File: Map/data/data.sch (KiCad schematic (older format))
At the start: 0 parts

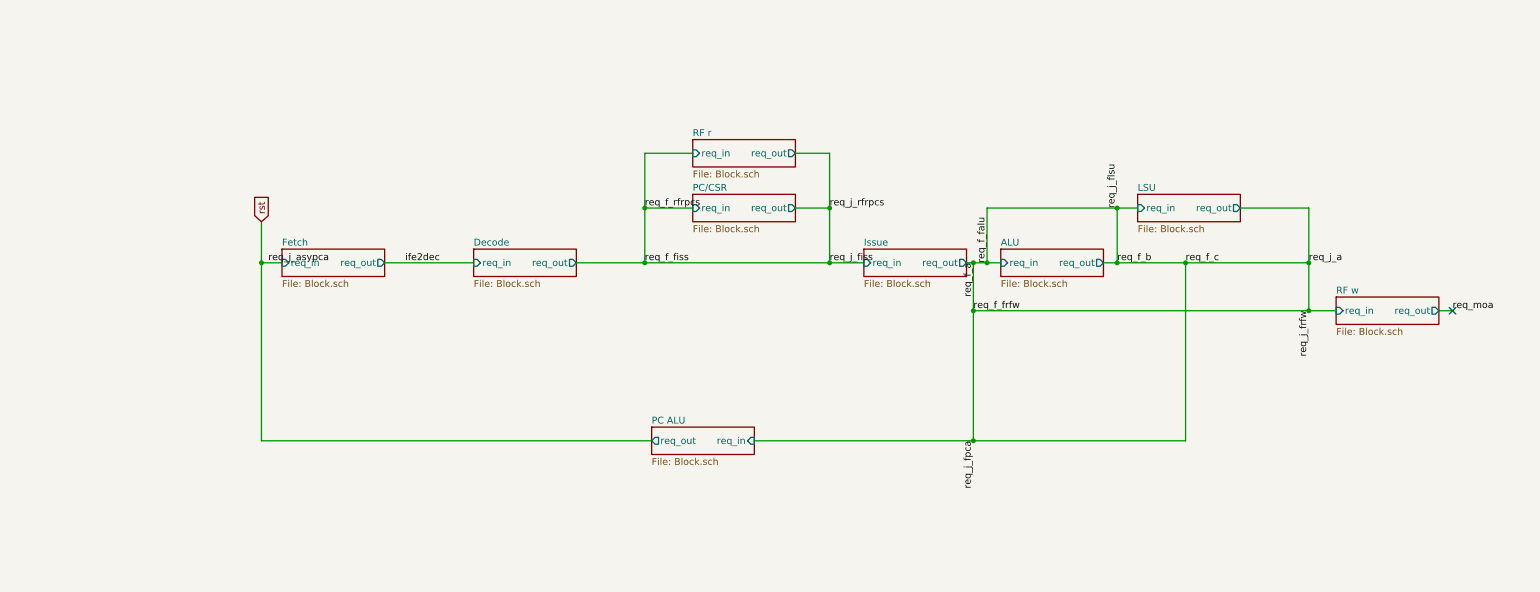
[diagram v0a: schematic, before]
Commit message: travail sur muller
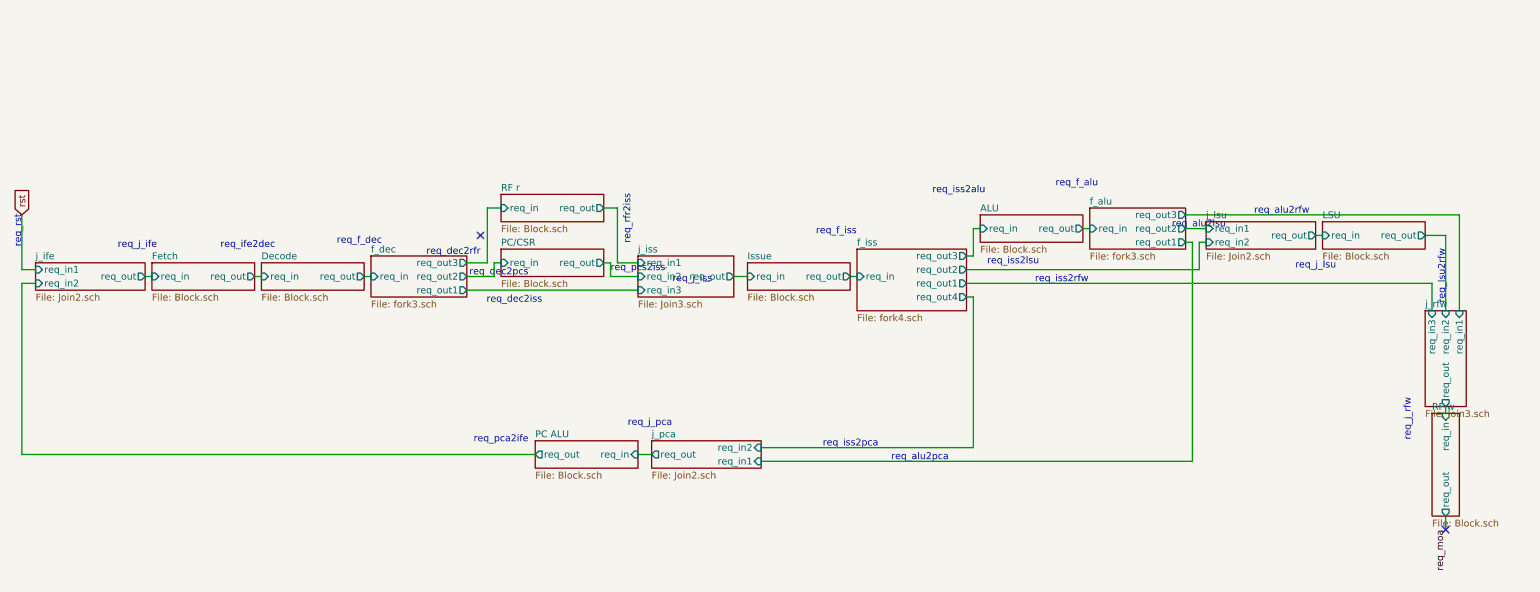
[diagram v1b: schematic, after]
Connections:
- no-connect marks 1 -> 2
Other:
- note added: "req_alu2lsu\n"
- note added: "req_alu2pca"
- note added: "req_alu2rfw\n"
- note added: "req_dec2iss\n"
- note added: "req_dec2pcs\n"
- note added: "req_dec2rfr\n"
- note added: "req_f_alu\n"
- note added: "req_f_dec\n\n"
- note added: "req_f_iss\n"
- note added: "req_ife2dec\n"
- note added: "req_iss2alu\n"
- note added: "req_iss2lsu\n\n"
- note added: "req_iss2pca\n"
- note added: "req_iss2rfw\n"
- note added: "req_j_ife\n"
- note added: "req_j_iss"
- note added: "req_j_lsu\n"
- note added: "req_j_pca\n"
- note added: "req_j_rfw\n"
- note added: "req_lsu2rfw\n"
- note added: "req_pca2ife\n\n"
- note added: "req_pcs2iss\n\n"
- note added: "req_rfr2iss"
- note added: "req_rst\n"

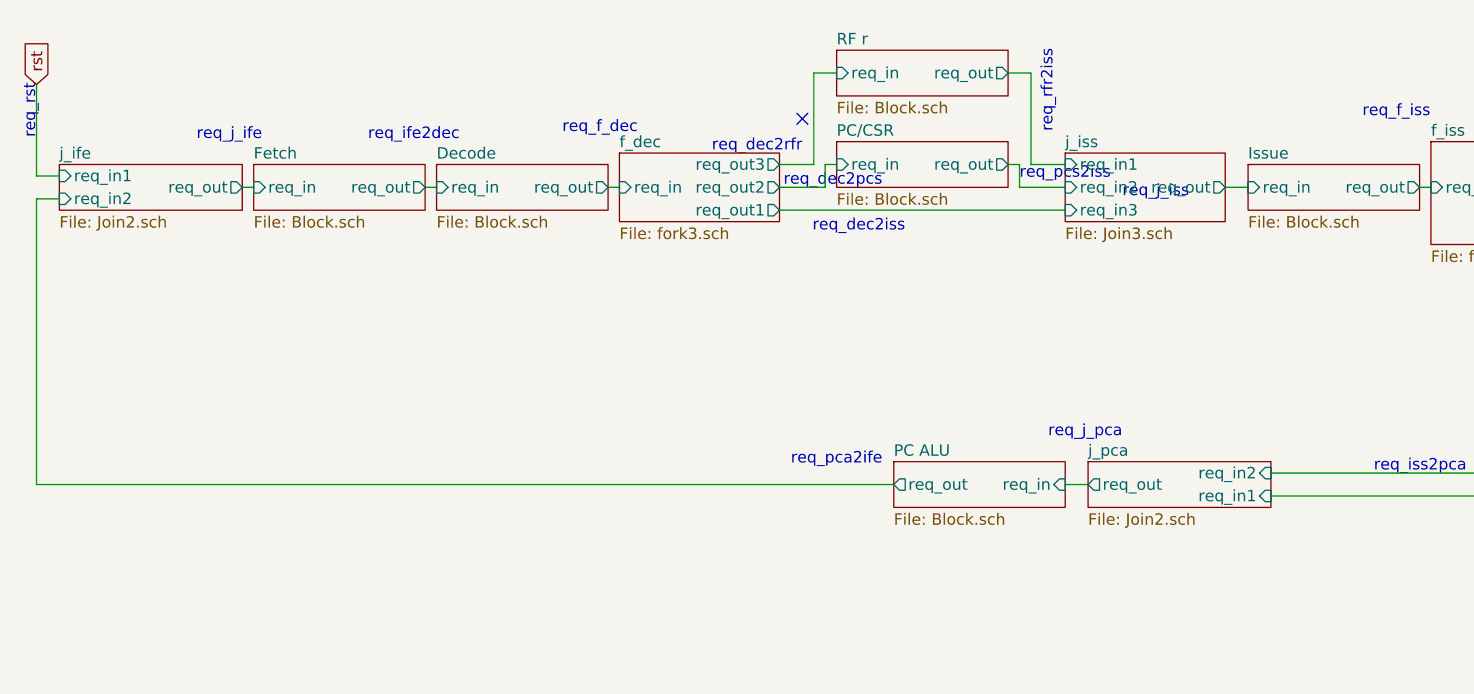
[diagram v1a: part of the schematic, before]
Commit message: Release v1
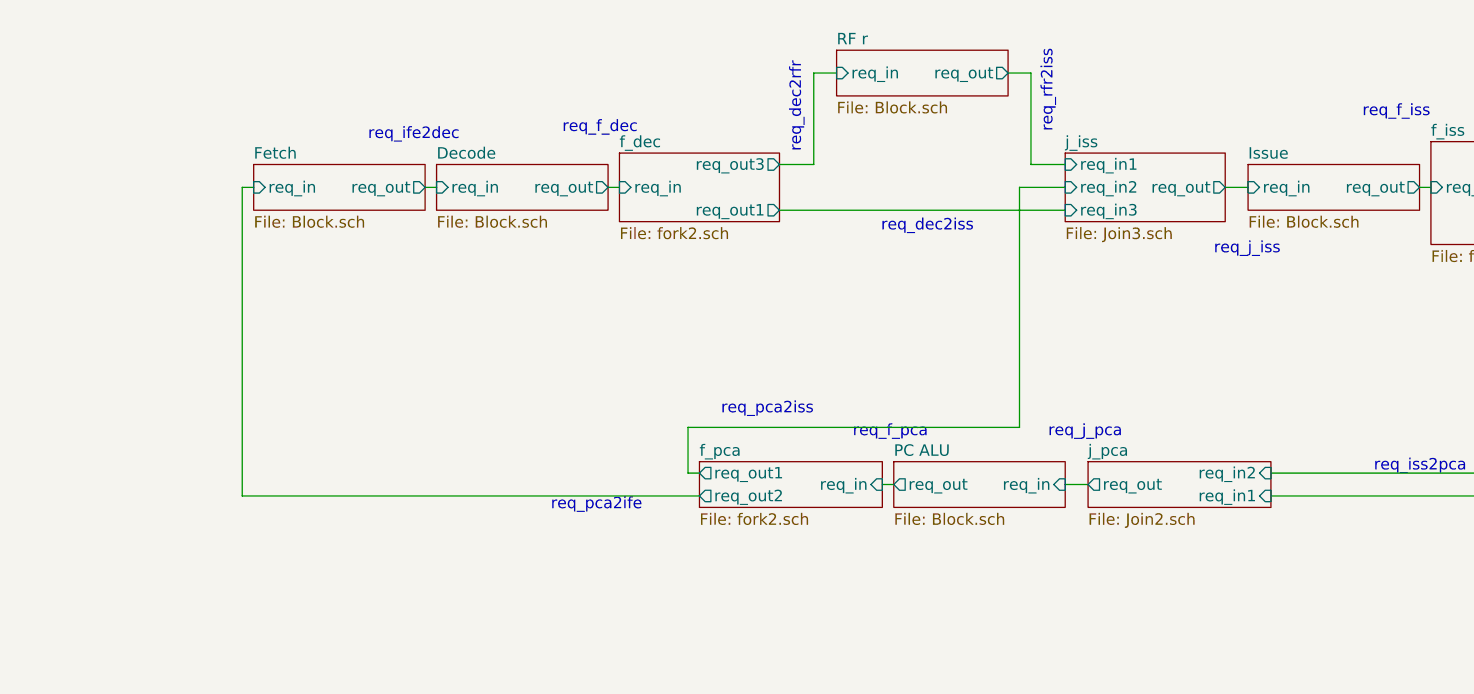
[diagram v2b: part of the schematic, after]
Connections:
- no-connect marks 2 -> 1
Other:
- note added: "req_f_pca"
- note added: "req_pca2iss\n"
- note removed: "req_dec2pcs\n"
- note removed: "req_j_ife\n"
- note removed: "req_pcs2iss\n\n"
- note removed: "req_rst\n"
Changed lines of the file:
@@
 $Descr A4 11693 8268
 encoding utf-8
-Sheet 1 18
+Sheet 1 17
 Title ""
 Date ""
@@
 $EndSheet
 $Sheet
-S 4050 2600 750  200
-U 5EAC82B1
-F0 "PC/CSR" 50
-F1 "Block.sch" 50
-F2 "req_in" I L 4050 2700 50
-F3 "req_out" O R 4800 2700 50
-$EndSheet
-$Sheet
 S 5850 2700 750  200
 U 5EAC8327
@@
 Wire Wire Line
 	1450 2800 1500 2800
-Text GLabel 550  2350 1    50   Input ~ 0
-rst
 Text Label 10950 4650 3    50   ~ 0
 req_moa
-$Sheet
-S 650  2700 800  200
-U 5EAD46D6
-F0 "j_ife" 50
-F1 "Join2.sch" 50
-F2 "req_out" O R 1450 2800 50
-F3 "req_in1" I L 650 2750 50
-F4 "req_in2" I L 650 2850 50
-$EndSheet
-Wire Wire Line
-	650  2750 550  2750
-Wire Wire Line
-	550  2350 550  2750
-Wire Wire Line
-	550  4100 550  2850
-Wire Wire Line
-	550  2850 650  2850
-Wire Wire Line
-	550  4100 4300 4100
 $Sheet
 S 5050 2650 700  300
@@
 F4 "req_in2" I L 5050 2800 50
 F5 "req_in3" I L 5050 2900 50
-$EndSheet
-$Sheet
-S 3100 2650 700  300
-U 5EAD914F
-F0 "f_dec" 50
-F1 "fork3.sch" 50
-F2 "req_in" I L 3100 2800 50
-F3 "req_out1" O R 3800 2900 50
-F4 "req_out2" O R 3800 2800 50
-F5 "req_out3" O R 3800 2700 50
 $EndSheet
 $Sheet
@@
 	5050 2900 3800 2900
 Wire Wire Line
-	3800 2800 4000 2800
-Wire Wire Line
-	4000 2800 4000 2700
-Wire Wire Line
-	4000 2700 4050 2700
-Wire Wire Line
-	4800 2700 4850 2700
-Wire Wire Line
-	4850 2700 4850 2800
-Wire Wire Line
 	4850 2800 5050 2800
 Wire Wire Line
@@
 Text Notes 2000 2600 0    50   ~ 0
 req_ife2dec\n
-Text Notes 1250 2600 0    50   ~ 0
-req_j_ife\n
 Text Notes 2850 2650 0    50   ~ 0
 req_f_dec\n\n
-Text Notes 3900 2650 2    50   ~ 0
-req_dec2rfr\n
-Text Notes 4250 2800 2    50   ~ 0
-req_dec2pcs\n
-Text Notes 4350 3000 2    50   ~ 0
+Text Notes 4650 3000 2    50   ~ 0
 req_dec2iss\n
 Text Notes 5000 2200 3    50   ~ 0
 req_rfr2iss
-Text Notes 4850 2850 0    50   ~ 0
-req_pcs2iss\n\n
 Wire Wire Line
 	4900 2700 5050 2700
-Text Notes 5300 2850 0    50   ~ 0
+Text Notes 5700 3100 0    50   ~ 0
 req_j_iss
 Text Notes 6350 2500 0    50   ~ 0
@@
 Text Notes 5300 3900 2    50   ~ 0
 req_j_pca\n
-Text Notes 4250 4100 2    50   ~ 0
+Text Notes 3200 4300 2    50   ~ 0
 req_pca2ife\n\n
-Text Notes 550  2350 3    50   ~ 0
-req_rst\n
 Text Notes 9850 2750 0    50   ~ 0
 req_j_lsu\n
-NoConn ~ 3900 2500
+$Sheet
+S 3450 4000 800  200
+U 5EB0D305
+F0 "f_pca" 50
+F1 "fork2.sch" 50
+F2 "req_in" I R 4250 4100 50
+F3 "req_out1" O L 3450 4050 50
+F4 "req_out2" O L 3450 4150 50
+$EndSheet
+Wire Wire Line
+	4300 4100 4250 4100
+Text Notes 4450 3900 2    50   ~ 0
+req_f_pca
+Wire Wire Line
+	3450 4150 1450 4150
+Wire Wire Line
+	1450 4150 1450 2800
+Text Notes 3900 2650 1    50   ~ 0
+req_dec2rfr\n
+$Sheet
+S 3100 2650 700  300
+U 5EAD914F
+F0 "f_dec" 50
+F1 "fork2.sch" 50
+F2 "req_in" I L 3100 2800 50
+F3 "req_out1" O R 3800 2900 50
+F4 "req_out3" O R 3800 2700 50
+$EndSheet
+Wire Wire Line
+	4850 2800 4850 3850
+Wire Wire Line
+	4850 3850 3400 3850
+Wire Wire Line
+	3400 3850 3400 4050
+Wire Wire Line
+	3400 4050 3450 4050
+Text Notes 3950 3800 2    50   ~ 0
+req_pca2iss\n
 $EndSCHEMATC

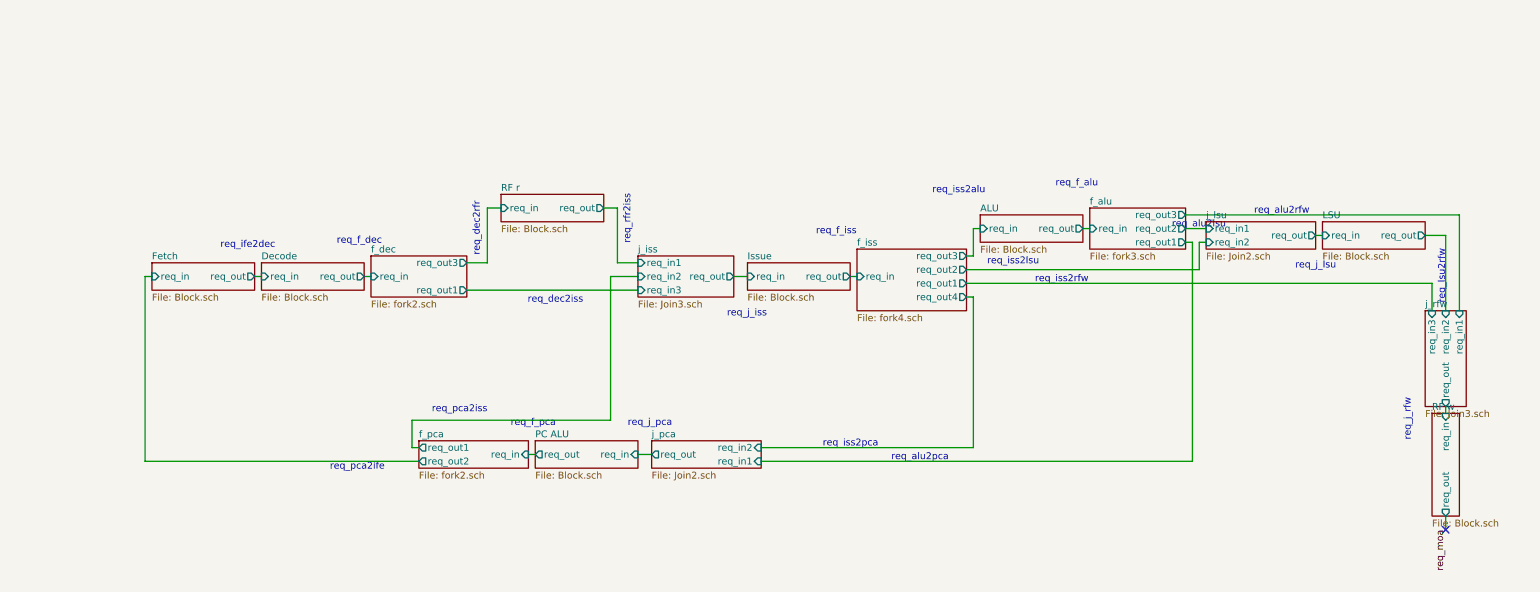
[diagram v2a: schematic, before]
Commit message: screen
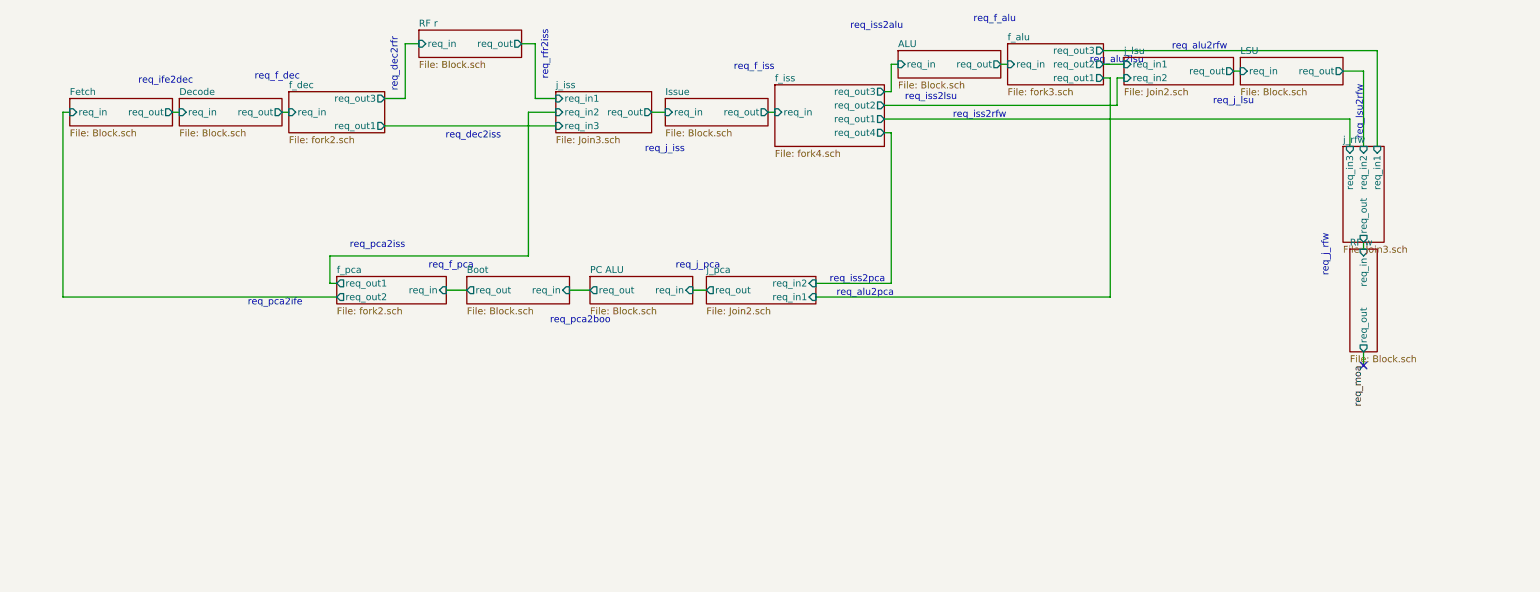
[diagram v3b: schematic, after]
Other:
- note added: "req_pca2boo\n"
